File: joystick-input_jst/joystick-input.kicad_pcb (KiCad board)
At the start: 2 copper layers, 71.4 x 38.9 mm, 38 parts, among them J11 Conn_01x05, J12 Conn_01x02, J13 Conn_01x02, J14 Conn_01x02, J15 Conn_01x02, J16 Conn_01x02, J17 Conn_01x02, J18 Conn_01x02, J19 Conn_01x02, J21 Conn_01x05, J22 Conn_01x02, J23 Conn_01x02, J24 Conn_01x02, J25 Conn_01x02, J26 Conn_01x02, J27 Conn_01x02, J28 Conn_01x02, J29 Conn_01x02

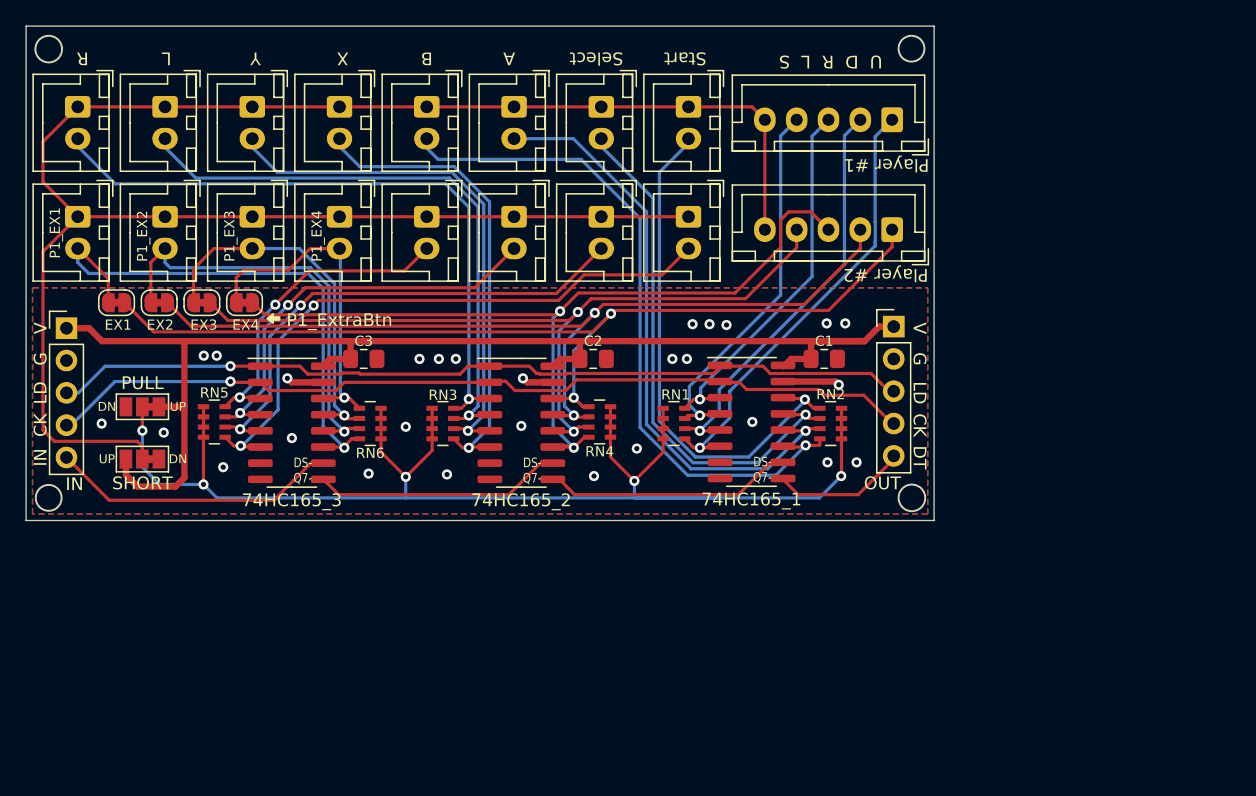
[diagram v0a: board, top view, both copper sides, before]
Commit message: 도면 시트 설명 추가
Signed-off-by: Ju, Gyeong-min <jcmh74@gmail.com>
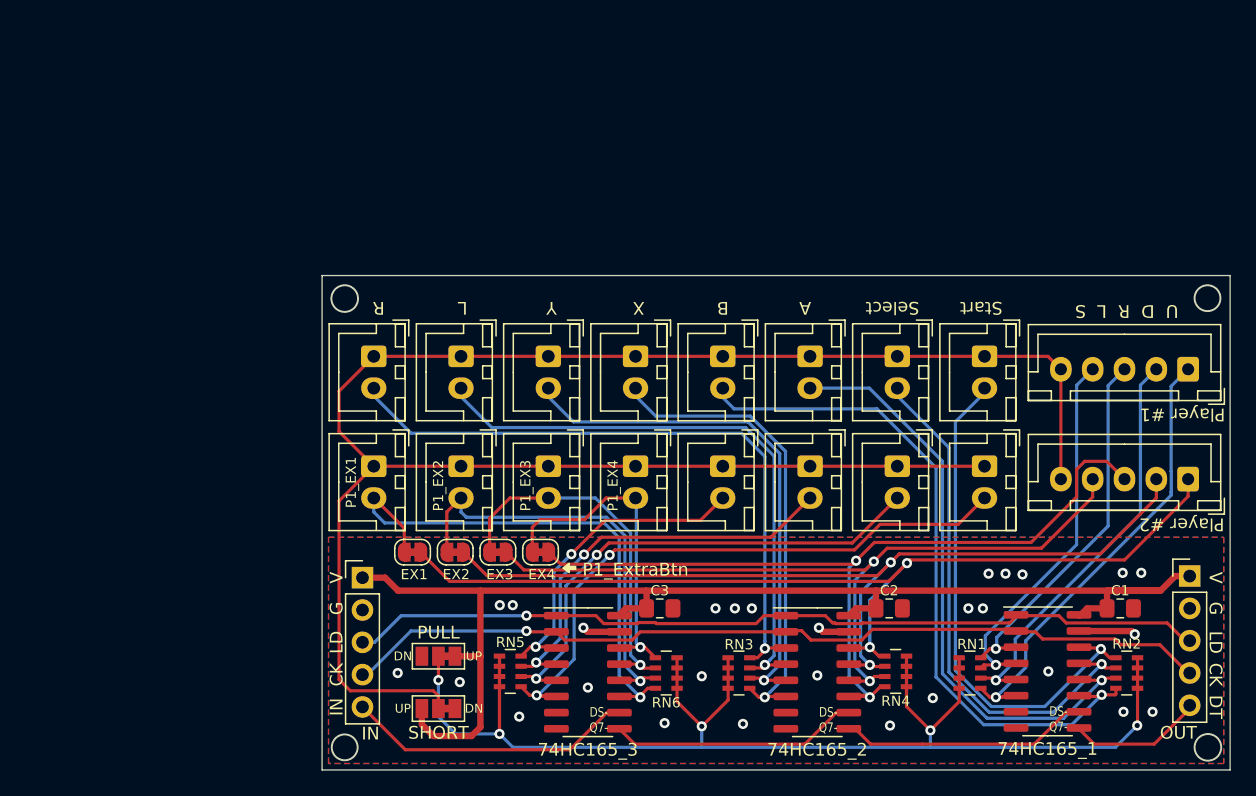
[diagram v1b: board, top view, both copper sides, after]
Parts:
- moved J25 30.4 mm to (148.5, 92.8)
- moved J15 30.4 mm to (148.5, 84.1)
- moved 74HC165_2 30.4 mm to (155.9, 109.0)
- moved 74HC165_3 30.4 mm to (137.9, 109.0)
- moved C1 30.4 mm to (179.7, 103.9)
- moved C2 30.4 mm to (161.6, 103.9)
- moved C3 30.4 mm to (143.5, 103.9)
- moved J11 30.4 mm to (185.1, 85.1)
- moved J22 30.4 mm to (169.1, 92.8)
- moved J23 30.4 mm to (162.2, 92.8)
- moved J26 30.4 mm to (141.6, 92.8)
- moved J27 30.4 mm to (134.8, 92.8)
- moved J28 30.4 mm to (127.9, 92.8)
- moved JP3 30.4 mm to (124.1, 99.5)
- moved JP4 30.4 mm to (127.5, 99.5)
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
